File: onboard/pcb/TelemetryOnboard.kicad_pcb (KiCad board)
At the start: 4 copper layers, 100 x 91 mm, 80 parts, among them J1 90 Deg. Socket 02x03 2.54mm, J2 Socket 01x02 2.54mm, J3 CONSMA001-SMD-G-T, J4 Socket 01x04 2.54mm, J5 Socket 01x02 2.54mm, U1 AVR128DB64x-xPT, U2 RC1780HP-RC232

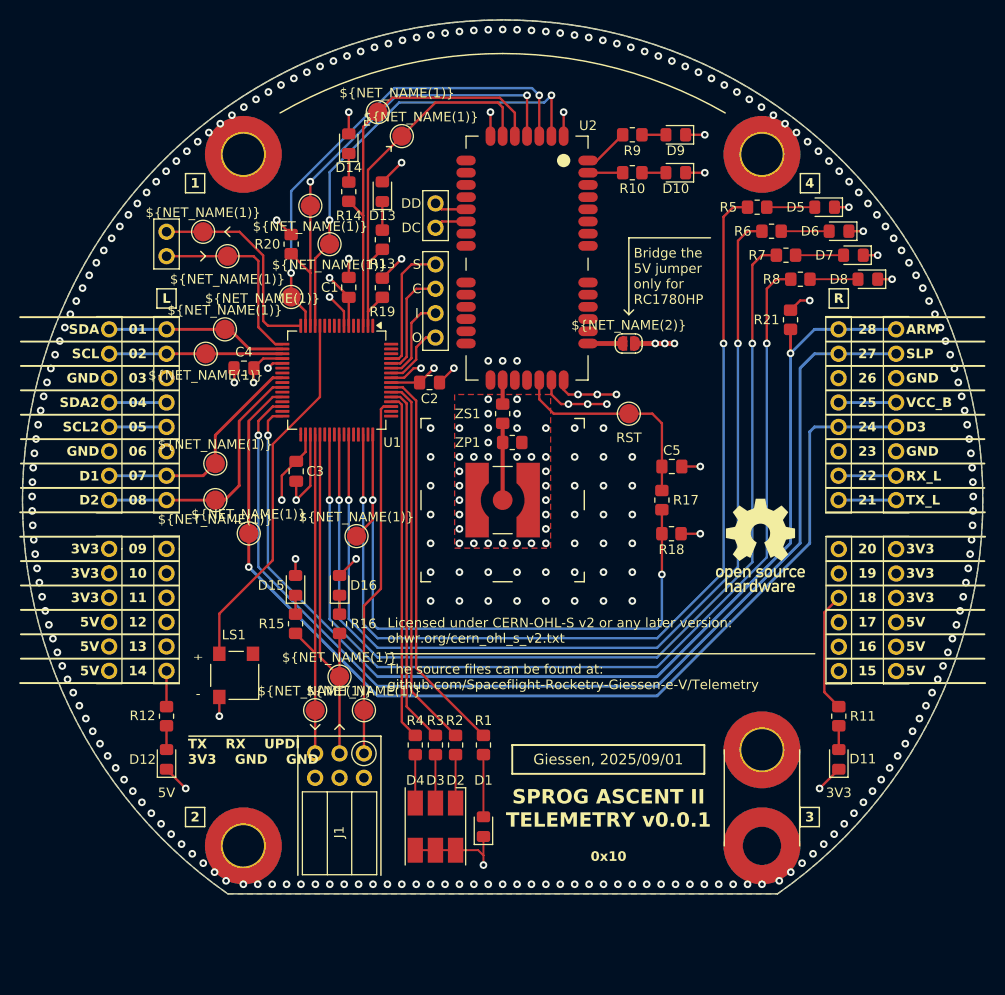
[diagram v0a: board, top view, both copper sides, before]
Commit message: first version new schematic
added symbols, footprints, 3dmodels, added new pcb base layout, added first schematic elements
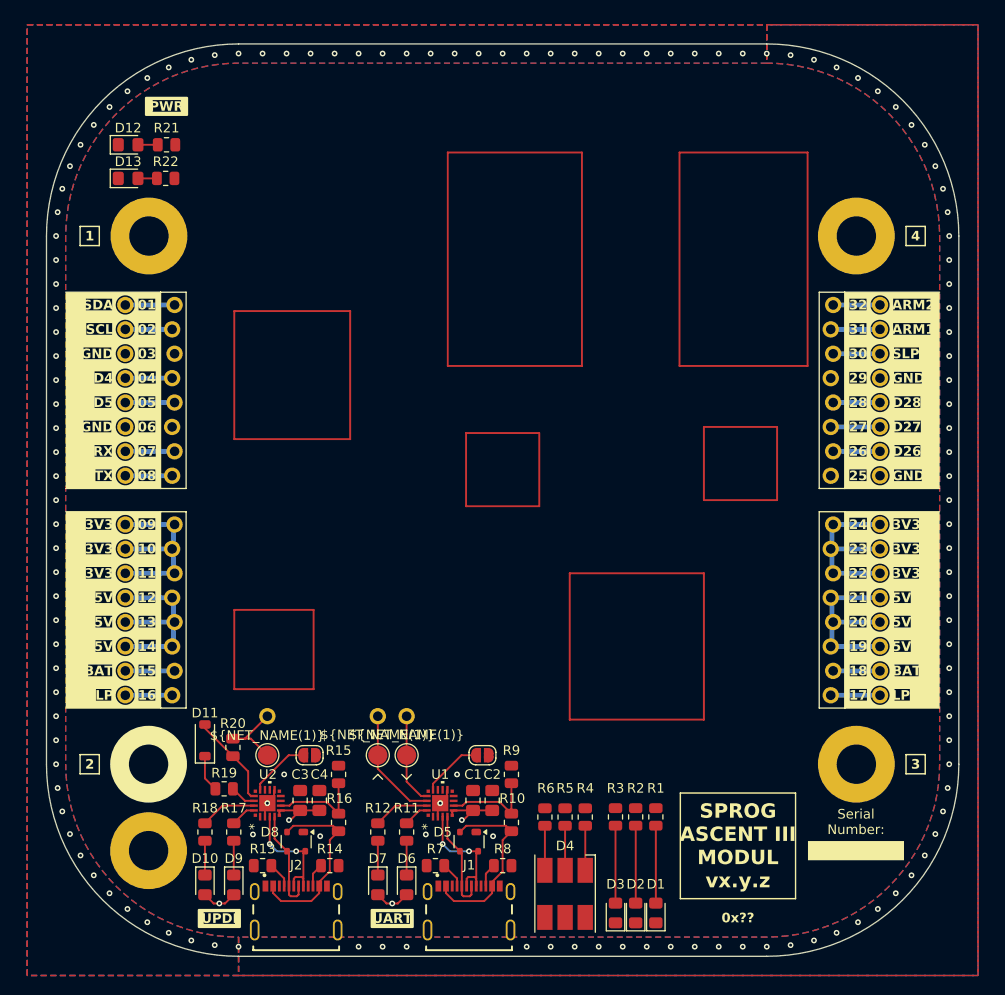
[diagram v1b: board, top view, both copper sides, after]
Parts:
- removed C5: 1nF, Capacitor_SMD:C_0805_2012Metric_Pad1.18x1.45mm_HandSolder
- removed D14, D15, D16: LED 0805 red, LED_SMD:LED_0805_2012Metric_Pad1.15x1.40mm_HandSolder
- removed J3: CONSMA001-SMD-G-T, Footprints:SMA Connector CONSMA001-SMD-G-T
- removed J4: Socket 01x04 2.54mm, Connector_PinSocket_2.54mm:PinSocket_1x04_P2.54mm_Vertical
- removed J5: Socket 01x02 2.54mm, Connector_PinSocket_2.54mm:PinSocket_1x02_P2.54mm_Vertical
- removed LS1: CMT-0525-75-SMT-TR, Footprints:Buzzer XDCR_CMT-0525-75-SMT-TR
- removed TP10, TP11, TP12, TP13, TP14, TP15, TP16, TP17, TP4, TP5, TP6, TP7, TP8, TP9: ~, Footprints:Test Point
- removed ZP1, ZS1: ~, Resistor_SMD:R_0805_2012Metric_Pad1.20x1.40mm_HandSolder
- added D3: orange, LED_SMD:LED_0805_2012Metric_Pad1.15x1.40mm_HandSolder, F.Cu at (11.8, 43.0)
- added D4: Cree RGB LED, Footprints:Cree RGB LED, F.Cu at (6.50, 41.0)
- added JP2: SolderJumper_2_Open, Footprints:Solder Jumper, F.Cu at (-20.1, 26.6)
- added R22: 560 Ohm, Resistor_SMD:R_0805_2012Metric, F.Cu at (-35.1, -33.5)
- added REF**: Test Point Hole, Footprints:Test Point Hole, F.Cu at (-24.5, 22.5)
- added REF**: Test Point Hole, Footprints:Test Point Hole, F.Cu at (-10.0, 22.5)
- added REF**: Test Point Hole, Footprints:Test Point Hole, F.Cu at (-13.0, 22.5)
- C1, C3: value 1uF -> 4.7 uF
- C2, C4: value 1uF -> 0.1 uF
- D1, D7: value LED 0805 orange -> orange
- D10: value LED 0805 green -> orange
- D11: value LED 0805 green -> BAT43; footprint LED_SMD:LED_0805_2012Metric_Pad1.15x1.40mm_HandSolder -> Diode_SMD:D_SOD-123
- D12: value LED 0805 green -> green
- D13: value LED 0805 red -> green
- D2: value CLS6B-FKW -> orange; footprint Footprints:RGB LED Cree-PLCC-6_6x5mm_P2.1mm -> LED_SMD:LED_0805_2012Metric_Pad1.15x1.40mm_HandSolder
- D5, D8: value LED 0805 orange -> SP0503BAHT; footprint LED_SMD:LED_0805_2012Metric_Pad1.15x1.40mm_HandSolder -> Package_TO_SOT_SMD:SOT-143
- D6: value LED 0805 orange -> green
- D9: value LED 0805 yellow -> green
- J1: value 90 Deg. Socket 02x03 2.54mm -> USB-C; footprint Connector_PinSocket_2.54mm:PinSocket_2x03_P2.54mm_Horizontal -> Footprints:GCT_USB4215-03-A_REVA
- J2: value Socket 01x02 2.54mm -> USB-C; footprint Connector_PinSocket_2.54mm:PinSocket_1x02_P2.54mm_Vertical -> Footprints:GCT_USB4215-03-A_REVA
- JL1: value Stackable Header 01x08 2.54mm -> Stackable Socket 1x8; footprint Connector_PinSocket_2.54mm:PinSocket_1x08_P2.54mm_Vertical -> Footprints:JL1
- JL2: value Stackable Header 01x06 2.54mm -> Stackable Socket 1x8; footprint Connector_PinSocket_2.54mm:PinSocket_1x06_P2.54mm_Vertical -> Footprints:JL2
- JL3: value ~ -> Stackable Socket 1x8; footprint Connector_PinSocket_2.54mm:PinSocket_1x08_P2.54mm_Vertical -> Footprints:JL3
- JL4: value ~ -> Stackable Socket 1x8; footprint Connector_PinSocket_2.54mm:PinSocket_1x06_P2.54mm_Vertical -> Footprints:JL4
- JP1: value ~ -> SolderJumper_2_Open
- JR1: value Stackable Header 01x08 2.54mm -> Stackable Socket 1x8; footprint Connector_PinSocket_2.54mm:PinSocket_1x08_P2.54mm_Vertical -> Footprints:JR1
- JR2: value Stackable Header 01x06 2.54mm -> Stackable Socket 1x8; footprint Connector_PinSocket_2.54mm:PinSocket_1x06_P2.54mm_Vertical -> Footprints:JR2
- JR3: value ~ -> Stackable Socket 1x8; footprint Connector_PinSocket_2.54mm:PinSocket_1x08_P2.54mm_Vertical -> Footprints:JR3
- JR4: value ~ -> Stackable Socket 1x8; footprint Connector_PinSocket_2.54mm:PinSocket_1x06_P2.54mm_Vertical -> Footprints:JR4
- M1, M2, M3, M4: value ~ -> M4 Mounting Hole
- R1, R11, R12, R2, R3, R4, R5, R6: value 270R -> 560 Ohm; footprint Resistor_SMD:R_0805_2012Metric_Pad1.20x1.40mm_HandSolder -> Resistor_SMD:R_0805_2012Metric
- R10: value 270R -> 22k; footprint Resistor_SMD:R_0805_2012Metric_Pad1.20x1.40mm_HandSolder -> Resistor_SMD:R_0805_2012Metric
- R13, R14: value 1k -> 5k1; footprint Resistor_SMD:R_0805_2012Metric_Pad1.20x1.40mm_HandSolder -> Resistor_SMD:R_0805_2012Metric
- R15: value 1k -> 47k; footprint Resistor_SMD:R_0805_2012Metric_Pad1.20x1.40mm_HandSolder -> Resistor_SMD:R_0805_2012Metric
- R16: value 1k -> 22k; footprint Resistor_SMD:R_0805_2012Metric_Pad1.20x1.40mm_HandSolder -> Resistor_SMD:R_0805_2012Metric
- R17: value 2k7 -> 560 Ohm; footprint Resistor_SMD:R_0805_2012Metric_Pad1.20x1.40mm_HandSolder -> Resistor_SMD:R_0805_2012Metric
- R18, R21: value 5k6 -> 560 Ohm; footprint Resistor_SMD:R_0805_2012Metric_Pad1.20x1.40mm_HandSolder -> Resistor_SMD:R_0805_2012Metric
- R19, R20: value 5k6 -> 470 Ohm; footprint Resistor_SMD:R_0805_2012Metric_Pad1.20x1.40mm_HandSolder -> Resistor_SMD:R_0805_2012Metric
- R7, R8: value 270R -> 5k1; footprint Resistor_SMD:R_0805_2012Metric_Pad1.20x1.40mm_HandSolder -> Resistor_SMD:R_0805_2012Metric
- R9: value 270R -> 47k; footprint Resistor_SMD:R_0805_2012Metric_Pad1.20x1.40mm_HandSolder -> Resistor_SMD:R_0805_2012Metric
- TP1, TP2, TP3: value ~ -> TestPoint
- U1: value AVR128DB64x-xPT -> CP2102N; footprint Package_QFP:TQFP-64_10x10mm_P0.5mm -> Footprints:QFN20_CP2102N_SIL
- U2: value RC1780HP-RC232 -> CP2102N; footprint Footprints:Radiocrafts RC1780HP-RC232 -> Footprints:QFN20_CP2102N_SIL
- moved D9 90.7 mm to (-28.0, 40.1), turned to -90 degrees
- moved D10 88.9 mm to (-31.0, 40.1), turned to -90 degrees
- moved D8 83.5 mm to (-21.5, 35.6), turned to -90 degrees
- moved D7 82.2 mm to (-13.0, 40.1), turned to -90 degrees
- moved D6 81.6 mm to (-10.0, 40.1), turned to -90 degrees
- moved U2 77.1 mm to (-24.5, 31.6), turned to 90 degrees
- moved J2 77.0 mm to (-21.5, 44.8)
- moved D5 75.7 mm to (-3.50, 35.6), turned to -90 degrees
- moved R7 73.3 mm to (-7.00, 38.1)
- moved R14 70.2 mm to (-18.0, 38.1), turned to 0 degrees
- moved R10 68.8 mm to (0.91, 33.6), turned to 90 degrees
- moved R8 68.5 mm to (0.00, 38.1), turned to 0 degrees
- moved R9 67.8 mm to (0.91, 28.6), turned to 90 degrees
- moved R21 67.5 mm to (-35.0, -37.0), turned to 180 degrees
- moved R5 66.6 mm to (6.50, 33.0), turned to -90 degrees
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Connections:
- net SCL2 renamed D5
- net SDA2 renamed D4
- C2 pad 1: GND -> +3V3
- C2 pad 2: +3V3 -> GND
- C4 pad 1: GND -> +3V3
- C4 pad 2: +3V3 -> GND
- D10 pad 1: GND -> Net-(D10-K)
- D10 pad 2: Net-(D10-A) -> +3V3
- D11 pad 1: GND -> Net-(D11-K)
- D13 pad 1: Net-(D13-K) -> GND
- D13 pad 2: +3V3 -> Net-(D13-A)
- D2 pad 1: Net-(D2-AR) -> GND
- D2 pad 2: Net-(D2-AG) -> Net-(D2-A)
- D5 pad 2: Net-(D5-A) -> VBUS1
- D6 pad 1: GND -> Net-(D6-K)
- D6 pad 2: Net-(D6-A) -> +3V3
- D7 pad 1: GND -> Net-(D7-K)
- D7 pad 2: Net-(D7-A) -> +3V3
- D8 pad 2: Net-(D8-A) -> VBUS2
- D9 pad 1: GND -> Net-(D9-K)
- D9 pad 2: Net-(D9-A) -> +3V3
- JL1 pad 1: SDA0 -> SDA
- JL1 pad 2: SCL0 -> SCL
- JL1 pad 7: D1 -> RX_BUS
- JL1 pad 8: D2 -> TX_BUS
- JL3 pad 1: SDA0 -> SDA
- JL3 pad 2: SCL0 -> SCL
- JL3 pad 7: D1 -> RX_BUS
- JL3 pad 8: D2 -> TX_BUS
- JP1 pad 2: +5V -> GND
- JR1 pad 25: VCC_B -> GND
- JR1 pad 26: GND -> D26
- JR1 pad 27: SLP -> D27
- JR1 pad 28: ARM -> D28
- JR2 pad 17: +5V -> +3V_LP
- JR2 pad 18: +3V3 -> +V_BATT
- JR2 pad 19: +3V3 -> +5V
- JR2 pad 20: +3V3 -> +5V
- JR3 pad 25: VCC_B -> GND
- JR3 pad 26: GND -> D26
- JR3 pad 27: SLP -> D27
- JR3 pad 28: ARM -> D28
- JR4 pad 17: +5V -> +3V_LP
- JR4 pad 18: +3V3 -> +V_BATT
- JR4 pad 19: +3V3 -> +5V
- JR4 pad 20: +3V3 -> +5V
- R1 pad 1: LED EV -> LED 1
- R10 pad 1: Net-(D10-A) -> VBUS1
- R10 pad 2: Net-(U2-D1) -> Net-(U1-VBUS)
- R11 pad 1: +3V3 -> Net-(D6-K)
- R11 pad 2: Net-(D11-A) -> Net-(U1-~{TXT}/GPIO.2)
- R12 pad 1: +5V -> Net-(D7-K)
- R12 pad 2: Net-(D12-A) -> Net-(U1-~{RXT}/GPIO.3)
- R13 pad 1: Net-(D13-K) -> Net-(J2-CC1)
- R13 pad 2: TX0 -> GND
- R14 pad 1: RX0 -> Net-(J2-CC2)
- R14 pad 2: Net-(D14-K) -> GND
- R15 pad 1: Net-(D15-K) -> Net-(U2-VBUS)
- R15 pad 2: TX4 -> GND
- R16 pad 1: RX4 -> VBUS2
- R16 pad 2: Net-(D16-K) -> Net-(U2-VBUS)
- R17 pad 1: Net-(U2-RESET) -> Net-(D9-K)
- R17 pad 2: RST -> Net-(U2-~{TXT}/GPIO.2)
- R18 pad 1: +3V3 -> Net-(D10-K)
- R18 pad 2: RST -> Net-(U2-~{RXT}/GPIO.3)
- R19 pad 1: +3V3 -> Net-(D11-K)
- R19 pad 2: TX0 -> Net-(U2-TXD)
- R2 pad 1: LED R -> LED 2
- R2 pad 2: Net-(D2-AR) -> Net-(D2-A)
- R20 pad 1: +3V3 -> UPDI
- R20 pad 2: CFG -> Net-(D11-A)
- R21 pad 1: ARM -> +3V3
- R21 pad 2: GND -> Net-(D12-A)
- R3 pad 1: LED G -> LED 3
- R3 pad 2: Net-(D2-AG) -> Net-(D3-A)
- R4 pad 1: LED B -> LED R
- R4 pad 2: Net-(D2-AB) -> Net-(D4-AR)
- R5 pad 1: Net-(D5-A) -> LED G
- R5 pad 2: Net-(U1-PF2) -> Net-(D4-AG)
- R6 pad 1: Net-(D6-A) -> LED B
- R6 pad 2: Net-(U1-PE7) -> Net-(D4-AB)
- R7 pad 1: Net-(D7-A) -> Net-(J1-CC1)
- R7 pad 2: Net-(U1-PE5) -> GND
- R8 pad 1: Net-(D8-A) -> Net-(J1-CC2)
- R8 pad 2: Net-(U1-PE3) -> GND
- R9 pad 1: Net-(D9-A) -> Net-(U1-VBUS)
- R9 pad 2: Net-(U2-D2) -> GND
- TP1 pad 1: RST -> RX
- TP2 pad 1: CFG -> TX
- TP3 pad 1: TX0 -> UPDI
- U1 pad 12: Net-(U1-PB4) -> GND
- U1 pad 13: CTS -> unconnected-(U1-~{WAKEUP}-Pad13)
- U1 pad 14: CFG -> unconnected-(U1-SUSPEND-Pad14)
- U1 pad 15: RTS -> Net-(JP1-A)
- U1 pad 16: TX1 -> unconnected-(U1-~{RTS}-Pad16)
- U1 pad 17: RX1 -> TX
- U1 pad 18: SDA0 -> RX
- U1 pad 19: SCL0 -> Net-(U1-~{RXT}/GPIO.3)
- U1 pad 2: TX0 -> unconnected-(U1-CLK/GPIO.0-Pad2)
- U1 pad 20: +3V3 -> Net-(U1-~{TXT}/GPIO.2)
- U1 pad 3: RX0 -> GND
- U1 pad 4: unconnected-(U1-PA6-Pad4) -> D+1
- U1 pad 5: unconnected-(U1-PA7-Pad5) -> D-1
- U1 pad 7: GND -> +3V3
- U1 pad 8: unconnected-(U1-PB0-Pad8) -> Net-(U1-VBUS)
- U2 pad 1: GND -> unconnected-(U2-RS485/GPIO.1-Pad1)
- U2 pad 10: GND -> unconnected-(U2-NC-Pad10)
- U2 pad 12: Net-(U2-RESET) -> GND
- U2 pad 13: +3V3 -> unconnected-(U2-~{WAKEUP}-Pad13)
- U2 pad 14: GND -> unconnected-(U2-SUSPEND-Pad14)
- U2 pad 15: unconnected-(U2-Pad15) -> Net-(JP2-A)
- U2 pad 17: unconnected-(U2-Pad17) -> Net-(D11-A)
- U2 pad 18: unconnected-(U2-Pad18) -> Net-(U2-TXD)
- U2 pad 19: Net-(J2-Pin_1) -> Net-(U2-~{RXT}/GPIO.3)
- U2 pad 2: CTS -> unconnected-(U2-CLK/GPIO.0-Pad2)
- U2 pad 20: Net-(J2-Pin_2) -> Net-(U2-~{TXT}/GPIO.2)
- U2 pad 21: unconnected-(U2-Pad21) -> GND
- U2 pad 3: RTS -> GND
- U2 pad 4: CFG -> D+2
- U2 pad 5: RX0 -> D-2
- U2 pad 6: TX0 -> +3V3
- U2 pad 7: GND -> +3V3
- U2 pad 8: GND -> Net-(U2-VBUS)
- U2 pad 9: Net-(U2-RF) -> unconnected-(U2-~{RST}-Pad9)
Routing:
- net ARM: track 116.1 -> 0.00 mm, vias 2 -> 0
- net D3: track 111.1 -> 0.00 mm, vias 1 -> 0
- net SLP: track 114.9 -> 4.87 mm, vias 1 -> 0
- net Net-(U1-PE3): track 102.4 -> 0.00 mm, vias 2 -> 0
- net Net-(U1-PE5): track 101.9 -> 0.00 mm, vias 2 -> 0
- net Net-(U1-PE7): track 101.3 -> 0.00 mm, vias 2 -> 0
- net Net-(U1-PF2): track 100.6 -> 0.00 mm, vias 2 -> 0
- net +5V: track 110.6 -> 38.1 mm, vias 3 -> 0
- net RST: track 66.6 -> 0.00 mm, vias 2 -> 0
- net GND: track 65.9 -> 6.25 mm, vias 296 -> 136
- net RTS: track 49.5 -> 0.00 mm, vias 2 -> 0
- net CFG: track 48.4 -> 0.00 mm, vias 2 -> 0
- net CTS: track 47.3 -> 0.00 mm, vias 2 -> 0
- net RX0: track 43.0 -> 0.00 mm
- net LED EV: track 40.9 -> 0.00 mm
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- removed copper zone on In2.Cu, net +3V3
- removed copper zone on In2.Cu, net +5V
- removed copper zone on In1.Cu, net GND
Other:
- board size 100 x 91 mm -> 95 x 95 mm
- copper layers 4 -> 2
- board text added: "0x??"
- board text added: "29"
- board text added: "30"
- board text added: "31"
- board text added: "32"
- board text added: "ARM1"
- board text added: "ARM2"
- board text added: "BAT"
- board text added: "D26"
- board text added: "D27"
- board text added: "D28"
- board text added: "D5"
- board text added: "LP"
- board text added: "PWR"
- board text added: "RX"
- board text added: "SPROG ASCENT III MODUL vx.y.z"
- board text added: "Serial Number:"
- board text added: "TX"
- board text added: "UART"
- board text added: "UPDI"
- board text removed: "0x10"
- board text removed: "ARM"
- board text removed: "Bridge the 5V jumper only for RC1780HP"
- board text removed: "C"
- board text removed: "D1"
- board text removed: "D2"
- board text removed: "D3"
- board text removed: "DC"
- board text removed: "DD"
- board text removed: "Giessen, 2025/09/01"
- board text removed: "I"
- board text removed: "JLCJLCJLCJLC"
- board text removed: "L"
- board text removed: "Licensed under CERN-OHL-S v2 or any later version: ohwr.org/cern_ohl_s_v2.txt The source files can be found at: github.com/Spaceflight-Rocketry-Giessen-e-V/Telemetry"
- board text removed: "O"
- board text removed: "R"
- board text removed: "RX_L"
- board text removed: "S"
- board text removed: "SCL2"
- board text removed: "SDA2"
- board text removed: "SPROG ASCENT II TELEMETRY v0.0.1"
- board text removed: "TX RX UPDI 3V3 GND GND"
- board text removed: "TX_L"
- board text removed: "UPDI RX TX GND GND 3V3"
- board text removed: "VCC_B"

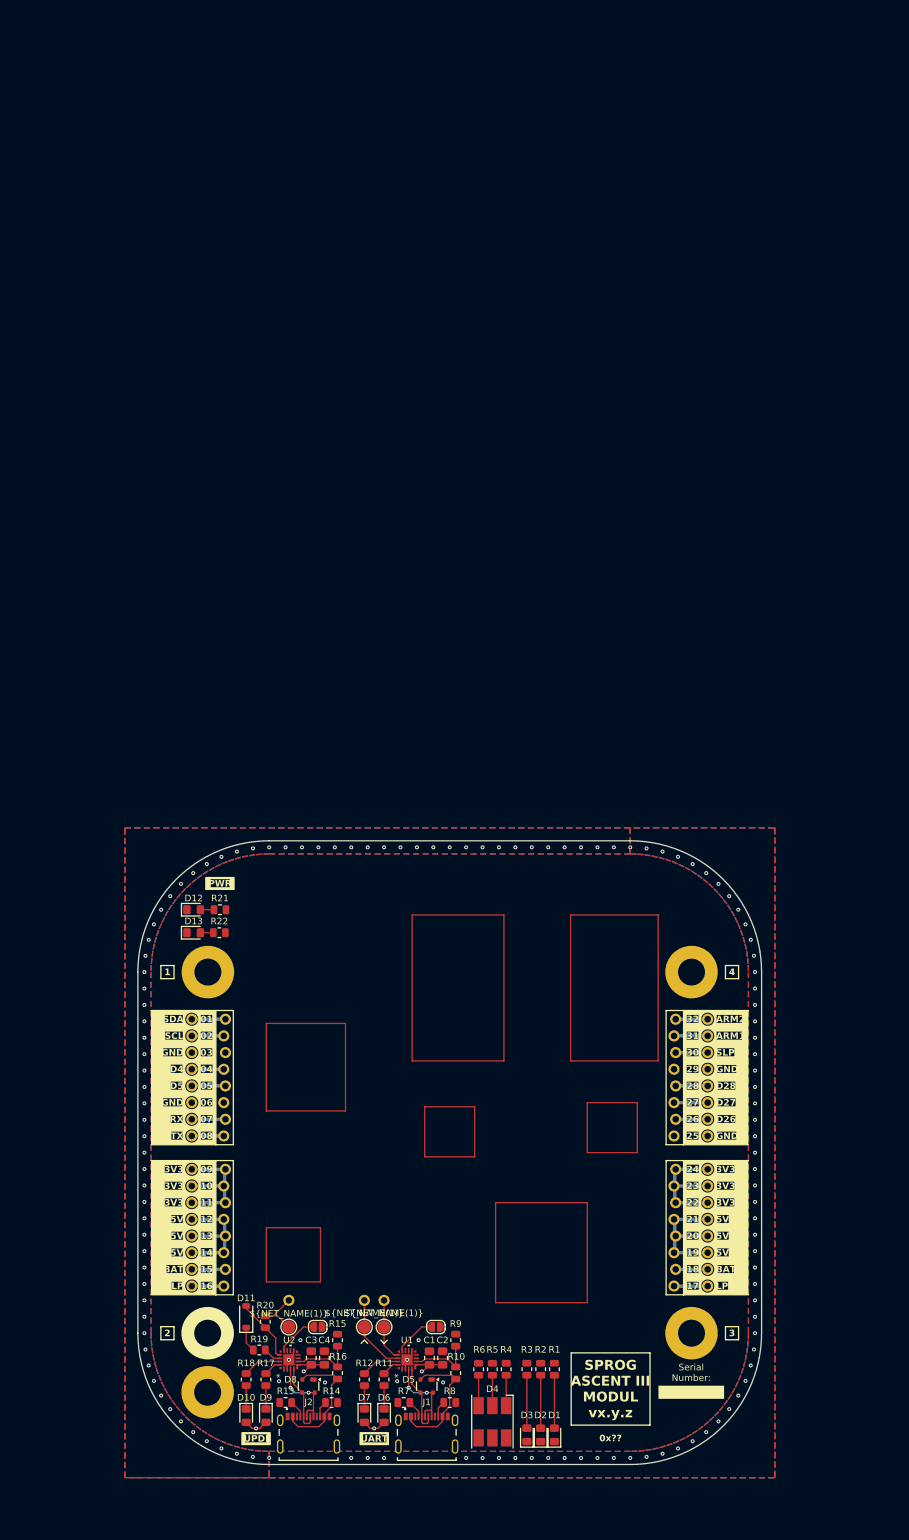
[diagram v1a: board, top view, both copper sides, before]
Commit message: update platine
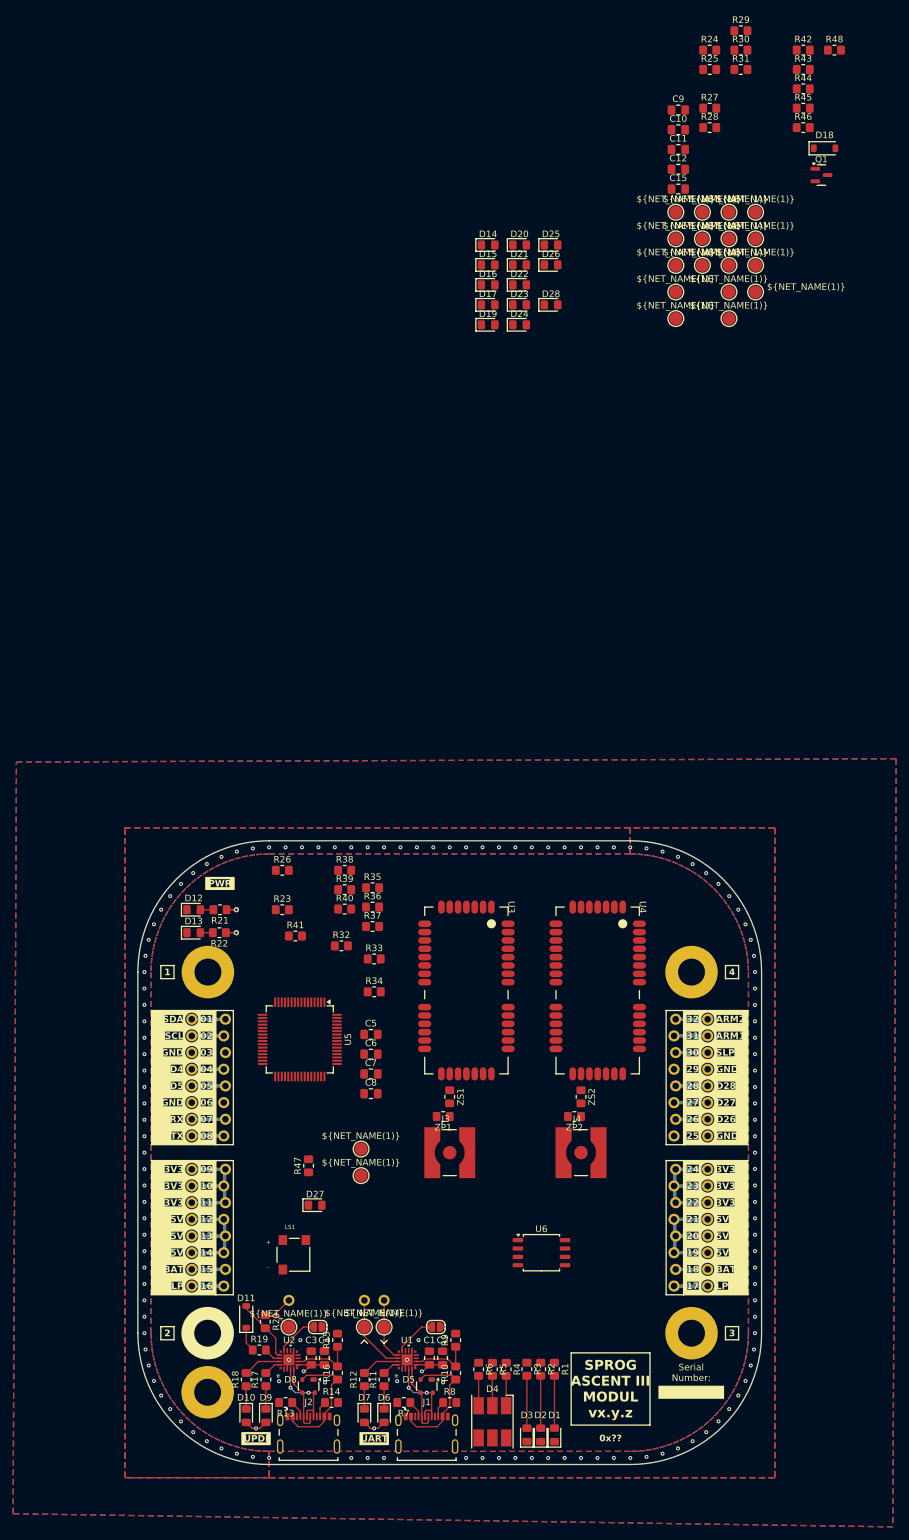
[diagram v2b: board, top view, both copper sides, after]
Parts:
- added C10: 0805 1uF, Capacitor_SMD:C_0805_2012Metric_Pad1.18x1.45mm_HandSolder, F.Cu at (34.8, -155.8)
- added C11: 0805 1uF, Capacitor_SMD:C_0805_2012Metric_Pad1.18x1.45mm_HandSolder, F.Cu at (34.8, -152.8)
- added C12: 0805 1uF, Capacitor_SMD:C_0805_2012Metric_Pad1.18x1.45mm_HandSolder, F.Cu at (34.8, -149.8)
- added C15: 1 uf, Capacitor_SMD:C_0805_2012Metric_Pad1.18x1.45mm_HandSolder, F.Cu at (34.8, -146.8)
- added C5: 0805 1nF, Capacitor_SMD:C_0805_2012Metric_Pad1.18x1.45mm_HandSolder, F.Cu at (-12.0, -18.0)
- added C6: 1 uf, Capacitor_SMD:C_0805_2012Metric_Pad1.18x1.45mm_HandSolder, F.Cu at (-12.0, -15.0)
- added C7: 0805 1nF, Capacitor_SMD:C_0805_2012Metric_Pad1.18x1.45mm_HandSolder, F.Cu at (-12.0, -12.0)
- added C8: 1 uf, Capacitor_SMD:C_0805_2012Metric_Pad1.18x1.45mm_HandSolder, F.Cu at (-12.0, -8.98)
- added C9: 0805 1uF, Capacitor_SMD:C_0805_2012Metric_Pad1.18x1.45mm_HandSolder, F.Cu at (34.8, -158.8)
- added D14: LED 0805 green, LED_SMD:LED_0805_2012Metric_Pad1.15x1.40mm_HandSolder, F.Cu at (5.84, -138.3)
- added D15: LED 0805 yellow, LED_SMD:LED_0805_2012Metric_Pad1.15x1.40mm_HandSolder, F.Cu at (5.84, -135.2)
- added D16: LED 0805 green, LED_SMD:LED_0805_2012Metric_Pad1.15x1.40mm_HandSolder, F.Cu at (5.84, -132.2)
- added D17: LED 0805 yellow, LED_SMD:LED_0805_2012Metric_Pad1.15x1.40mm_HandSolder, F.Cu at (5.84, -129.1)
- added D18: D, Diode_SMD:D_SOD-123, F.Cu at (57.1, -153.0)
- added D19: LED 0805 red, LED_SMD:LED_0805_2012Metric_Pad1.15x1.40mm_HandSolder, F.Cu at (5.84, -126.1)
- added D20: LED 0805 red, LED_SMD:LED_0805_2012Metric_Pad1.15x1.40mm_HandSolder, F.Cu at (10.6, -138.3)
- added D21: LED 0805 red, LED_SMD:LED_0805_2012Metric_Pad1.15x1.40mm_HandSolder, F.Cu at (10.6, -135.2)
- added D22: LED 0805 red, LED_SMD:LED_0805_2012Metric_Pad1.15x1.40mm_HandSolder, F.Cu at (10.6, -132.2)
- added D23: LED 0805 red, LED_SMD:LED_0805_2012Metric_Pad1.15x1.40mm_HandSolder, F.Cu at (10.6, -129.1)
- added D24: LED 0805 red, LED_SMD:LED_0805_2012Metric_Pad1.15x1.40mm_HandSolder, F.Cu at (10.6, -126.1)
- added D25: LED 0805 orange, LED_SMD:LED_0805_2012Metric_Pad1.15x1.40mm_HandSolder, F.Cu at (15.4, -138.3)
- added D26: LED 0805 orange, LED_SMD:LED_0805_2012Metric_Pad1.15x1.40mm_HandSolder, F.Cu at (15.4, -135.2)
- added D27: LED 0805 orange, LED_SMD:LED_0805_2012Metric_Pad1.15x1.40mm_HandSolder, F.Cu at (-20.5, 8.00)
- added D28: LED 0805 orange, LED_SMD:LED_0805_2012Metric_Pad1.15x1.40mm_HandSolder, F.Cu at (15.4, -129.1)
- added J3: CONSMA001-SMD-G-T, Footprints:SMA Connector CONSMA001-SMD-G-T, F.Cu at (0.00, 0.00)
- added J4: CONSMA001-SMD-G-T, Footprints:SMA Connector CONSMA001-SMD-G-T, F.Cu at (20.0, 0.00)
- added LS1: Buzzer CMT-0525-75-SMT-TR, Footprints:Buzzer XDCR_CMT-0525-75-SMT-TR, F.Cu at (-23.8, 15.6)
- added Q1: NPN, Package_TO_SOT_SMD:SOT-23, F.Cu at (56.6, -148.9)
- added R23: 0805 2k7, Resistor_SMD:R_0805_2012Metric_Pad1.20x1.40mm_HandSolder, F.Cu at (-25.5, -37.0)
- added R24: 0805 270R, Resistor_SMD:R_0805_2012Metric_Pad1.20x1.40mm_HandSolder, F.Cu at (39.6, -167.9)
- added R25: 0805 270R, Resistor_SMD:R_0805_2012Metric_Pad1.20x1.40mm_HandSolder, F.Cu at (39.6, -165.0)
- added R26: 0805 2k7, Resistor_SMD:R_0805_2012Metric_Pad1.20x1.40mm_HandSolder, F.Cu at (-25.5, -43.0)
- added R27: 0805 270R, Resistor_SMD:R_0805_2012Metric_Pad1.20x1.40mm_HandSolder, F.Cu at (39.6, -159.1)
- added R28: 0805 270R, Resistor_SMD:R_0805_2012Metric_Pad1.20x1.40mm_HandSolder, F.Cu at (39.6, -156.1)
- added R29: 180 R, Resistor_SMD:R_0805_2012Metric_Pad1.20x1.40mm_HandSolder, F.Cu at (44.3, -170.9)
- added R30: 10kR, Resistor_SMD:R_0805_2012Metric_Pad1.20x1.40mm_HandSolder, F.Cu at (44.3, -167.9)
- added R31: 10kR, Resistor_SMD:R_0805_2012Metric_Pad1.20x1.40mm_HandSolder, F.Cu at (44.3, -165.0)
- added R32: 0805 1k, Resistor_SMD:R_0805_2012Metric_Pad1.20x1.40mm_HandSolder, F.Cu at (-16.5, -31.5)
- added R33: 0805 1k, Resistor_SMD:R_0805_2012Metric_Pad1.20x1.40mm_HandSolder, F.Cu at (-11.5, -29.5)
- added R34: 0805 5k6, Resistor_SMD:R_0805_2012Metric_Pad1.20x1.40mm_HandSolder, F.Cu at (-11.5, -24.5)
- added R35: 0805 1k, Resistor_SMD:R_0805_2012Metric_Pad1.20x1.40mm_HandSolder, F.Cu at (-11.8, -40.4)
- added R36: 0805 1k, Resistor_SMD:R_0805_2012Metric_Pad1.20x1.40mm_HandSolder, F.Cu at (-11.8, -37.4)
- added R37: 0805 5k6, Resistor_SMD:R_0805_2012Metric_Pad1.20x1.40mm_HandSolder, F.Cu at (-11.8, -34.5)
- added R38: 0805 5k6, Resistor_SMD:R_0805_2012Metric_Pad1.20x1.40mm_HandSolder, F.Cu at (-16.0, -43.0)
- added R39: 0805 5k6, Resistor_SMD:R_0805_2012Metric_Pad1.20x1.40mm_HandSolder, F.Cu at (-16.0, -40.0)
- added R40: 0805 5k6, Resistor_SMD:R_0805_2012Metric_Pad1.20x1.40mm_HandSolder, F.Cu at (-16.0, -37.1)
- added R41: 0805 5k6, Resistor_SMD:R_0805_2012Metric_Pad1.20x1.40mm_HandSolder, F.Cu at (-23.5, -33.0)
- added R42: 5.6kR, Resistor_SMD:R_0805_2012Metric_Pad1.20x1.40mm_HandSolder, F.Cu at (53.8, -167.9)
- added R43: 0805 1k, Resistor_SMD:R_0805_2012Metric_Pad1.20x1.40mm_HandSolder, F.Cu at (53.8, -165.0)
- added R44: 0805 1k, Resistor_SMD:R_0805_2012Metric_Pad1.20x1.40mm_HandSolder, F.Cu at (53.8, -162.0)
- added R45: 0805 270R, Resistor_SMD:R_0805_2012Metric_Pad1.20x1.40mm_HandSolder, F.Cu at (53.8, -159.1)
- added R46: 0805 270R, Resistor_SMD:R_0805_2012Metric_Pad1.20x1.40mm_HandSolder, F.Cu at (53.8, -156.1)
- added R47: 0805 270R, Resistor_SMD:R_0805_2012Metric_Pad1.20x1.40mm_HandSolder, F.Cu at (-21.5, 2.00)
- added R48: 0805 270R, Resistor_SMD:R_0805_2012Metric_Pad1.20x1.40mm_HandSolder, F.Cu at (58.6, -167.9)
- added TP12: TestPoint, Footprints:Test Point, F.Cu at (34.4, -127.0)
- added TP13: TestPoint, Footprints:Test Point, F.Cu at (38.5, -143.2)
- added TP14: TestPoint, Footprints:Test Point, F.Cu at (38.5, -139.2)
- added TP15: TestPoint, Footprints:Test Point, F.Cu at (38.5, -135.1)
- added TP16: ~, Footprints:Test Point, F.Cu at (-13.5, -0.55)
- added TP17: ~, Footprints:Test Point, F.Cu at (-13.5, 3.50)
- added TP18: TestPoint, Footprints:Test Point, F.Cu at (42.5, -143.2)
- added TP19: TestPoint, Footprints:Test Point, F.Cu at (42.5, -139.2)
- added TP36: TestPoint, Footprints:Test Point, F.Cu at (42.5, -135.1)
- added TP37: TestPoint, Footprints:Test Point, F.Cu at (42.5, -131.1)
- added TP38: TestPoint, Footprints:Test Point, F.Cu at (42.5, -127.0)
- added TP39: TestPoint, Footprints:Test Point, F.Cu at (46.6, -143.2)
- added TP4: TestPoint, Footprints:Test Point, F.Cu at (34.4, -143.2)
- added TP40: ~, Footprints:Test Point, F.Cu at (46.6, -139.2)
- added TP41: TestPoint, Footprints:Test Point, F.Cu at (46.6, -135.1)
- added TP42: ~, Footprints:Test Point, F.Cu at (46.6, -131.1)
- added TP5: TestPoint, Footprints:Test Point, F.Cu at (34.4, -139.2)
- added TP8: TestPoint, Footprints:Test Point, F.Cu at (34.4, -135.1)
- added TP9: TestPoint, Footprints:Test Point, F.Cu at (34.4, -131.1)
- added U3: RC1780HP-RC232, Footprints:Radiocrafts RC1780HP-RC232, F.Cu at (8.89, -37.4)
- added U4: RC1701HP-RC232, Footprints:Radiocrafts RC1780HP-RC232, F.Cu at (28.9, -37.4)
- added U5: AVR128DB64x-xPT, Package_QFP:TQFP-64_10x10mm_P0.5mm, F.Cu at (-22.8, -17.2)
- added U6: W25Q80DVSSIG, Package_SO:SOIC-8_5.3x5.3mm_P1.27mm, F.Cu at (14.0, 15.2)
- added ZP1: ~, Resistor_SMD:R_0805_2012Metric_Pad1.20x1.40mm_HandSolder, F.Cu at (-1.00, -5.50)
- added ZP2: ~, Resistor_SMD:R_0805_2012Metric_Pad1.20x1.40mm_HandSolder, F.Cu at (19.0, -5.50)
- added ZS1: ~, Resistor_SMD:R_0805_2012Metric_Pad1.20x1.40mm_HandSolder, F.Cu at (0.00, -8.50)
- added ZS2: ~, Resistor_SMD:R_0805_2012Metric_Pad1.20x1.40mm_HandSolder, F.Cu at (20.0, -8.50)
- R1, R10, R11, R12, R13, R14, R15, R16, R17, R18, R19, R2, R20, R21, R22, R3, R4, R5, R6, R7, R8, R9: footprint Resistor_SMD:R_0805_2012Metric -> Resistor_SMD:R_0805_2012Metric_Pad1.20x1.40mm_HandSolder
- TP2, TP3: value TestPoint -> ~
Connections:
- net SCL renamed SCL1
- net SDA renamed SDA1
- TP1 pad 1: RX -> RST1
- TP2 pad 1: TX -> TX0
- TP3 pad 1: UPDI -> RX0
- U1 pad 17: TX -> TX4
- U1 pad 18: RX -> RX4
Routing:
- net +5V: track 38.1 -> 39.7 mm, vias 0 -> 1
- net +3V3: track 57.9 -> 59.4 mm, vias 4 -> 5
- added copper zone on In2.Cu, net +3V3
- added copper zone on In1.Cu, net GND
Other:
- copper layers 2 -> 4
